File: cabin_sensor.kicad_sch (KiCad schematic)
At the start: 6 parts, among them J5 Внутр. коннектор вентилятора 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, Q2 AO3400

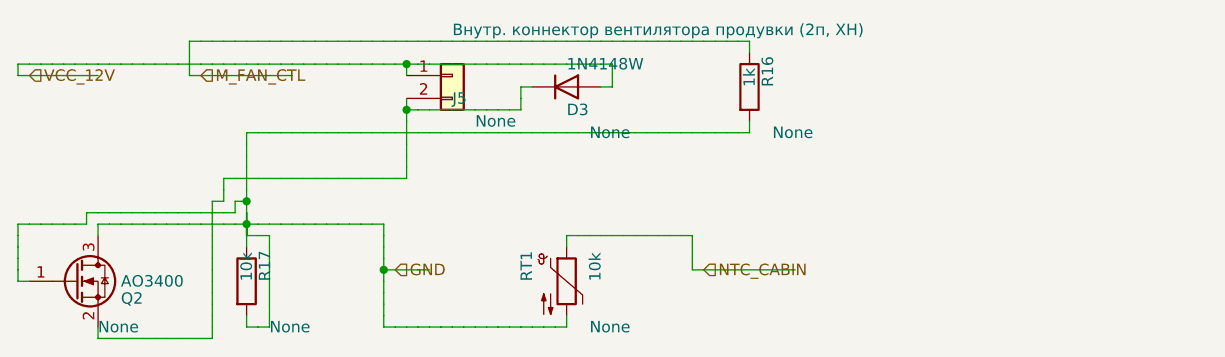
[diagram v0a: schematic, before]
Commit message: fix writer
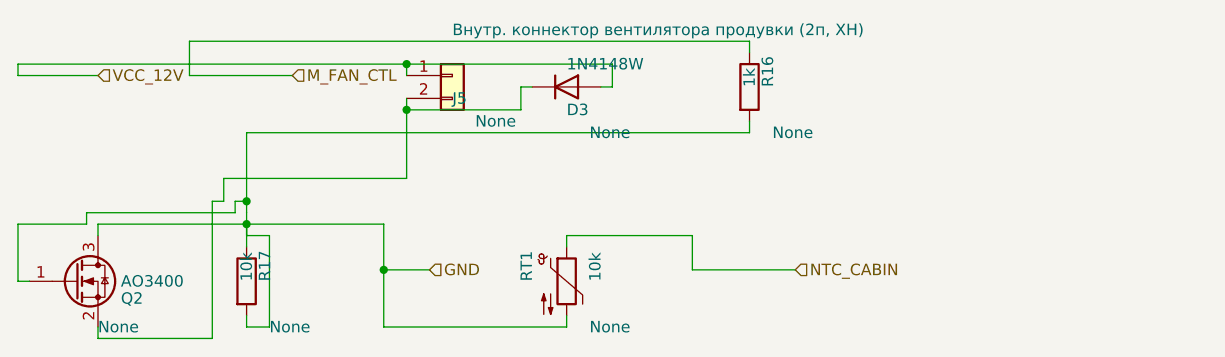
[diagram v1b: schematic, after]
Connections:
- net GND: no longer D3.1 (K), J5.2 (Pin_2), Q2.2 (S)
- net M_FAN_CTL: no longer D3.2 (A), J5.1 (Pin_1)
- new net: D3.1 (K), J5.2 (Pin_2), Q2.2 (S)
- new net VCC_12V: D3.2 (A), J5.1 (Pin_1)
